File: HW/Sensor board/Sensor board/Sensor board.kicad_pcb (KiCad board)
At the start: 2 copper layers, 66.5 x 47.5 mm, 22 parts, among them J1 RJ45_Shielded, U1 Hc-SR04, U2 DS92LV010A, U3 DS92LV010A, U4 LM2937xMP

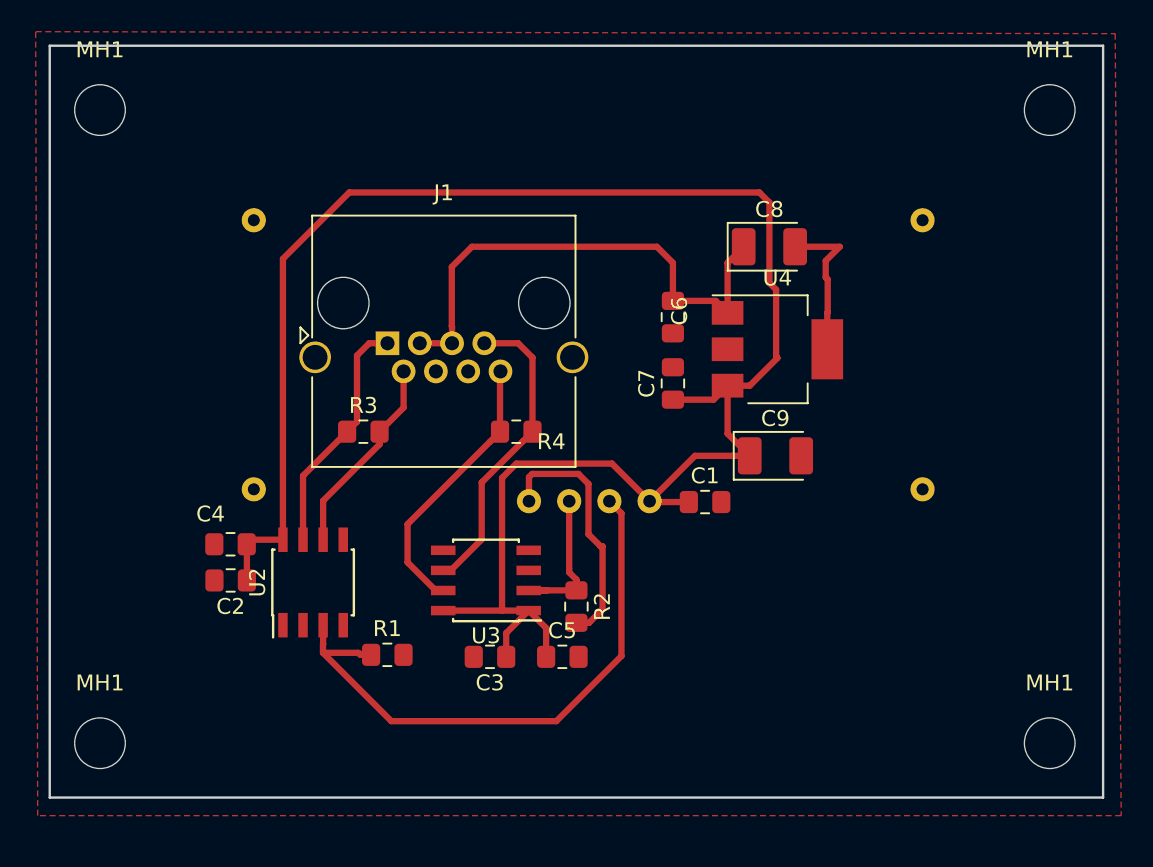
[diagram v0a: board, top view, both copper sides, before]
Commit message: fix
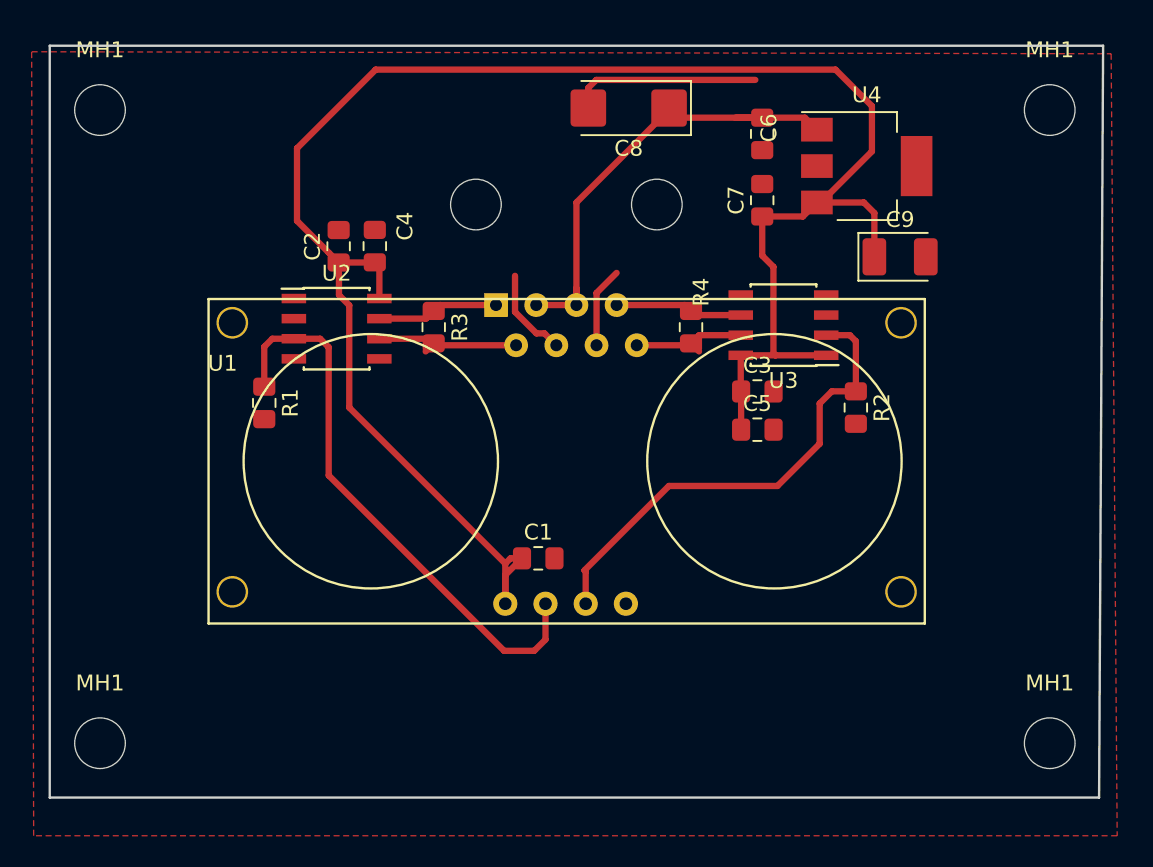
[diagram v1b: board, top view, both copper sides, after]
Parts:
- C8: footprint Capacitor_Tantalum_SMD:CP_EIA-3528-12_Kemet-T_Pad1.50x2.35mm_HandSolder -> Capacitor_Tantalum_SMD:CP_EIA-6032-20_AVX-F_Pad2.25x2.35mm_HandSolder
- J1: value RJ45_Shielded -> 8P8C; footprint Connector_RJ:RJ45_Amphenol_RJHSE5380 -> Connector_RJ:RJ45_Amphenol_54602-x08_Horizontal; moved to B.Cu
- U1: moved to F.Cu
- moved U1 47.1 mm to (117.0, 61.7), turned to 0 degrees
- moved U3 24.8 mm to (153.3, 63.4)
- moved C3 23.8 mm to (151.6, 67.6), turned to 0 degrees
- moved C2 22.2 mm to (125.2, 58.4), turned to 90 degrees
- moved R2 21.7 mm to (157.9, 68.6)
- moved C4 20.9 mm to (127.5, 58.4), turned to 90 degrees
- moved C5 18.9 mm to (151.6, 70.0)
- moved R1 17.7 mm to (120.5, 68.3), turned to 270 degrees
- moved U2 16.1 mm to (125.1, 63.6), turned to 0 degrees
- moved C9 14.8 mm to (160.7, 59.1)
- moved C6 12.9 mm to (151.9, 51.3)
- moved U4 12.9 mm to (158.5, 53.3)
- moved C7 12.9 mm to (151.9, 55.5)
- moved R4 12.9 mm to (147.4, 63.5), turned to 90 degrees
- moved C8 12.5 mm to (143.5, 49.7), turned to 180 degrees
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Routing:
- net ECHO: track 10.0 -> 30.7 mm
- net ECHO-: track 19.5 -> 8.10 mm
- net ECHO+: track 17.5 -> 7.55 mm
- net TRIG+: track 15.3 -> 7.73 mm
- net TRIG-: track 12.7 -> 9.53 mm
- net +12V: track 32.6 -> 29.6 mm
- net GND: track 25.7 -> 22.9 mm
- net TRIG: track 37.3 -> 36.0 mm
- net VCC: track 119.6 -> 120.6 mm
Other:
- outline, holes or cut-outs redrawn
